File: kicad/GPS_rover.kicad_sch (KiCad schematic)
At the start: 15 parts, among them J201 SMA, J202 NormallyClosed, U201 ZED_F9R, Y401 ANN-MB-00

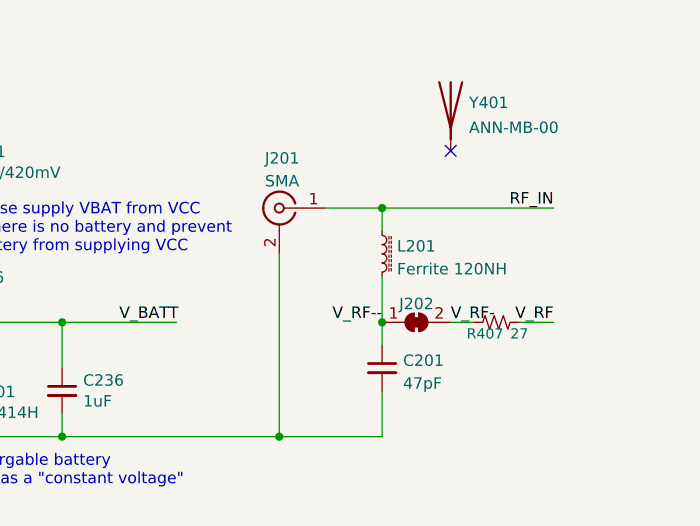
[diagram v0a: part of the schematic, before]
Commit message: Updated to KiCad 7.0
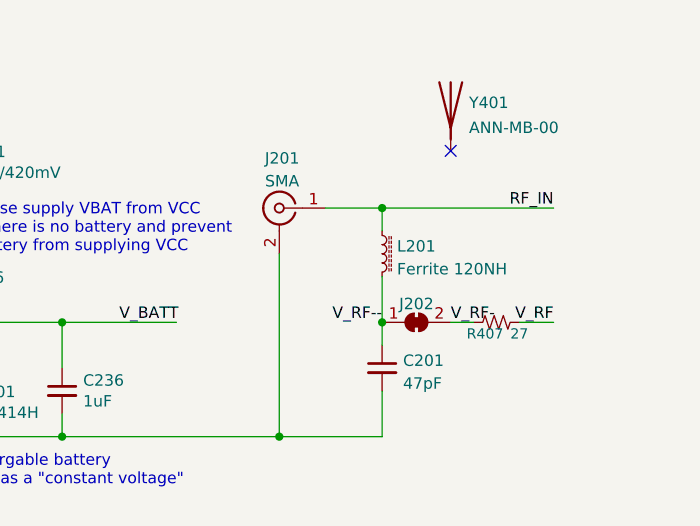
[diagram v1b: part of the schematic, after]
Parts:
- J201: Number in cart 1 -> (none); Number on hand 0 -> 1
